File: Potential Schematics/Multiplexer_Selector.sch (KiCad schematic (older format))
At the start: 6 parts, among them U269 74LS04, U28 74LS08, U281 74LS32, U290 74LS08, U291 74LS08, U292 74LS32

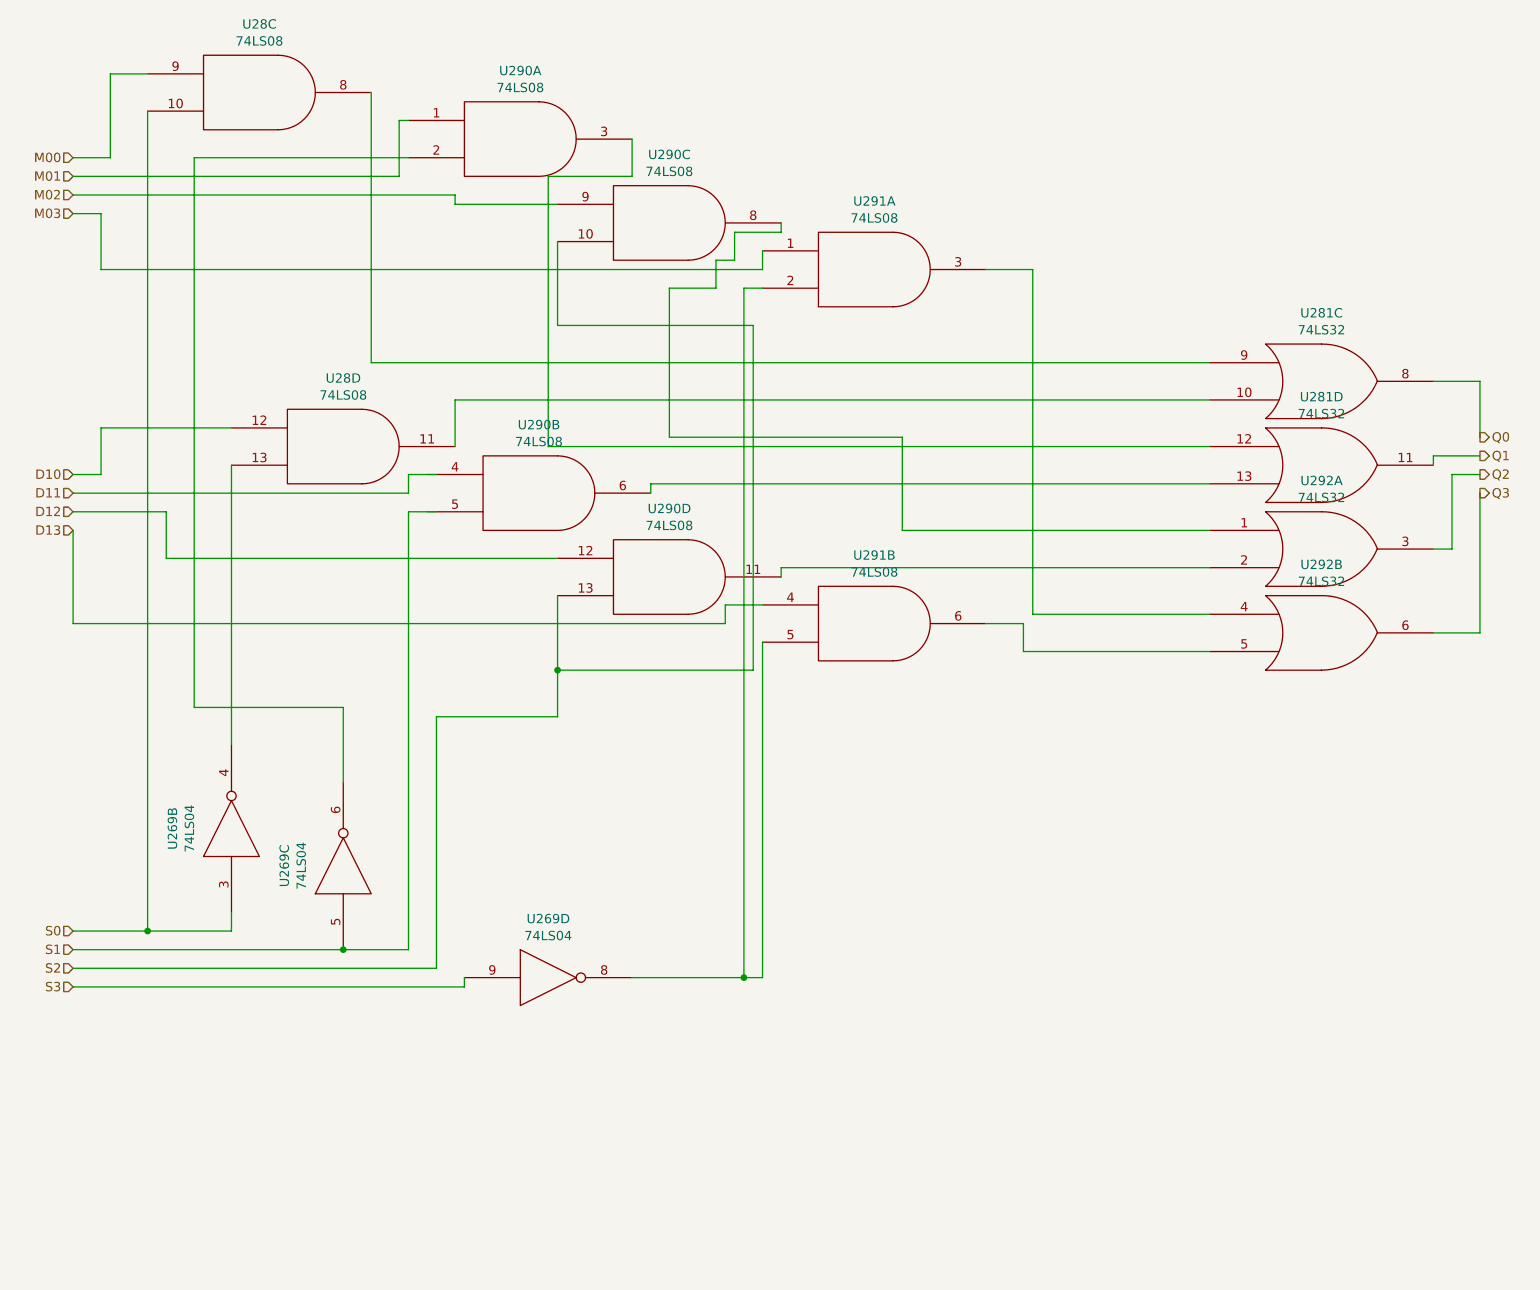
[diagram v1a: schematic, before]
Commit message: Made Multiplier
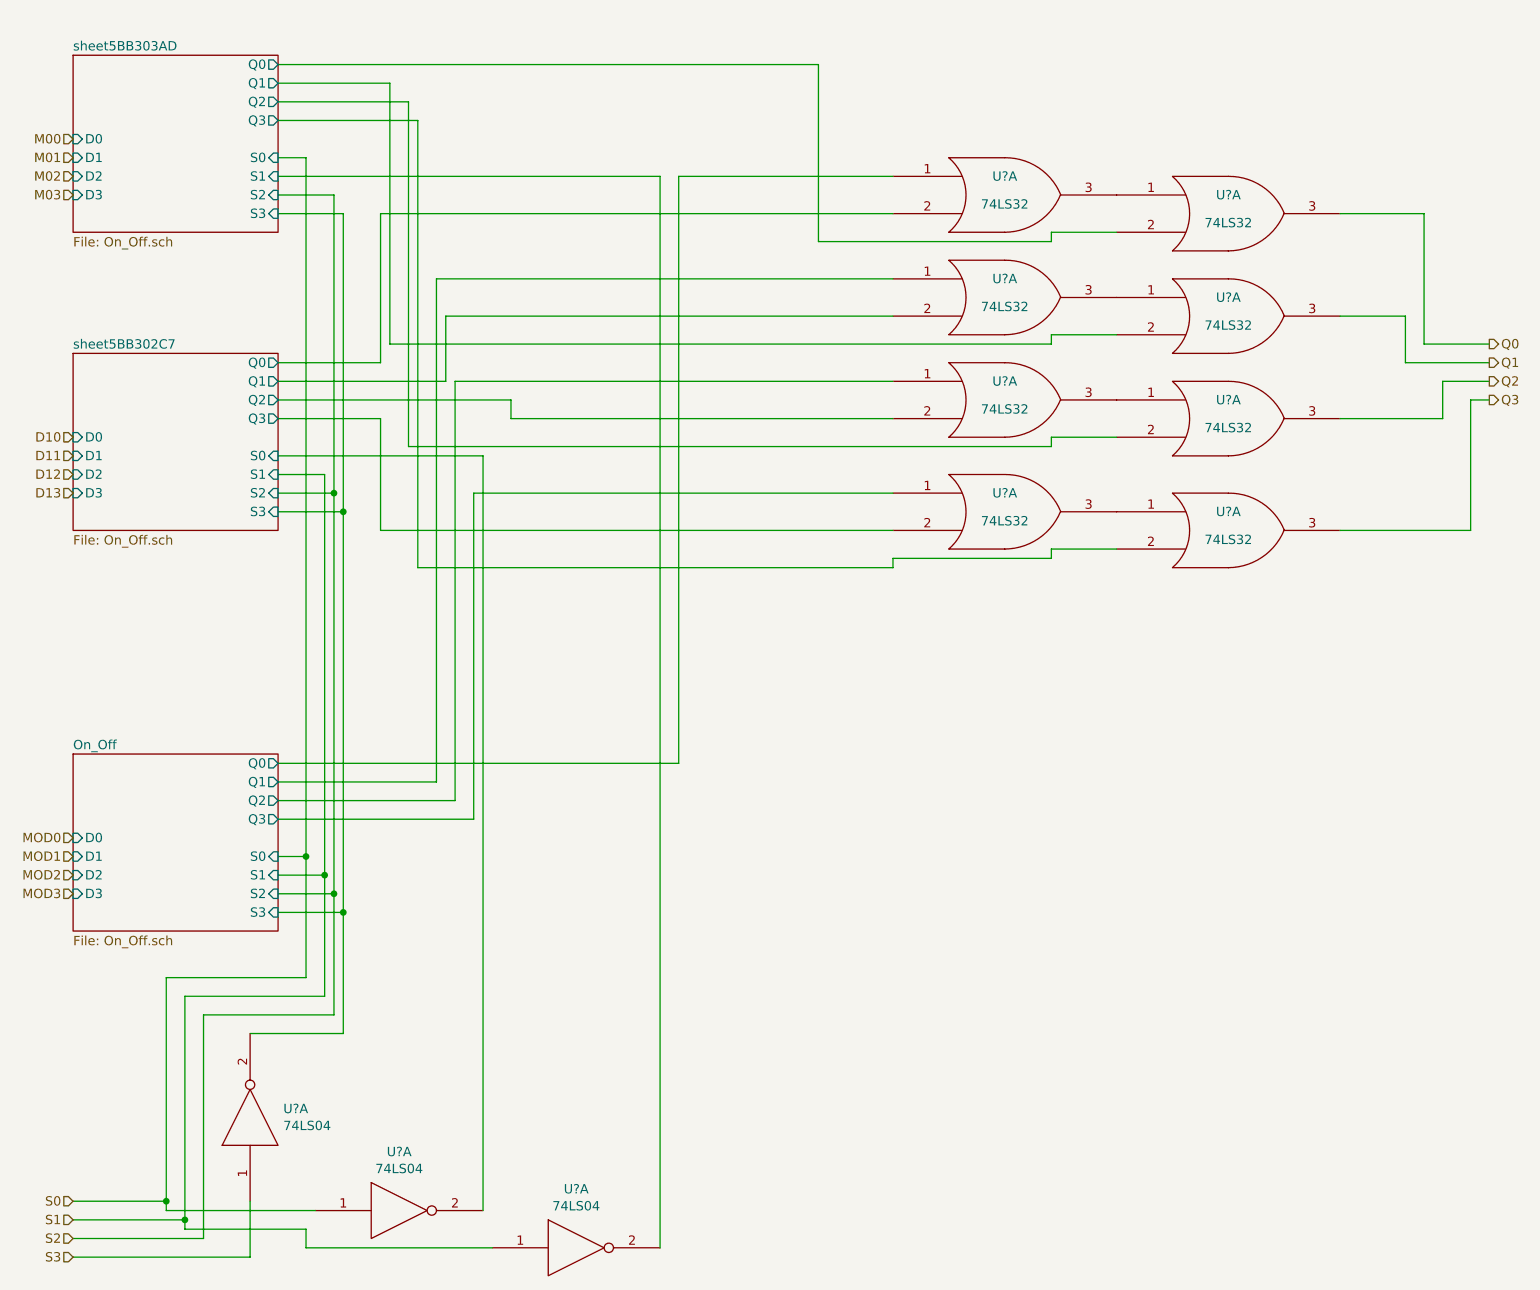
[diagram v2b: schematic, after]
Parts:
- removed U269: 74LS04, Daniel_Kopp:DIP-14_300_ELL, symbol 4-bit_processor-rescue:74LS04
- removed U28, U290, U291: 74LS08, Daniel_Kopp:DIP-14_300_ELL, symbol 4-bit_processor-rescue:74LS08
- removed U281, U292: 74LS32, Daniel_Kopp:DIP-14_300_ELL, symbol 4-bit_processor-rescue:74LS32
- added U? (x3): 74LS04, symbol 4-bit_processor-rescue:74LS04
- added U? (x8): 74LS32, symbol 4-bit_processor-rescue:74LS32
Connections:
- net GND: now also U?.7 (GND), U?.7 (GND), U?.7 (GND), U?.7 (GND), U?.7 (GND), U?.7 (GND), U?.7 (GND), U?.7 (GND), U?.7 (GND), U?.7 (GND), U?.7 (GND)
- net Q0: now also U?.3
- net Q1: now also U?.3
- net Q2: now also U?.3
- net Q3: now also U?.3
- net S0: now also U?.1
- net S1: now also U?.1
- net S3: now also U?.1
- net VCC: now also U?.14 (VCC), U?.14 (VCC), U?.14 (VCC), U?.14 (VCC), U?.14 (VCC), U?.14 (VCC), U?.14 (VCC), U?.14 (VCC), U?.14 (VCC), U?.14 (VCC), U?.14 (VCC)
- new net: U?.1, U?.3 (x4)
- new net On_Off/Q0: U?.1
- new net On_Off/Q1: U?.1
- new net On_Off/Q2: U?.1
- new net On_Off/Q3: U?.1
- new net On_Off/S3: U?.2
- new net sheet5BB302C7/Q0: U?.2
- new net sheet5BB302C7/Q1: U?.2
- new net sheet5BB302C7/Q2: U?.2
- new net sheet5BB302C7/Q3: U?.2
- new net sheet5BB302C7/S0: U?.2
- new net sheet5BB303AD/Q0: U?.2
- new net sheet5BB303AD/Q1: U?.2
- new net sheet5BB303AD/Q2: U?.2
- new net sheet5BB303AD/Q3: U?.2
- new net sheet5BB303AD/S1: U?.2
